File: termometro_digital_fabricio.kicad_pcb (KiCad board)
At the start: 2 copper layers, 100 x 100 mm, 30 parts, among them J1 Conn_01x01_Pin, SW1 SW_Push, U1 MT3608, U2 L7805, U3 LM35-LP, U4 ICL7107CPL, U5 ICL7660, U7 18650

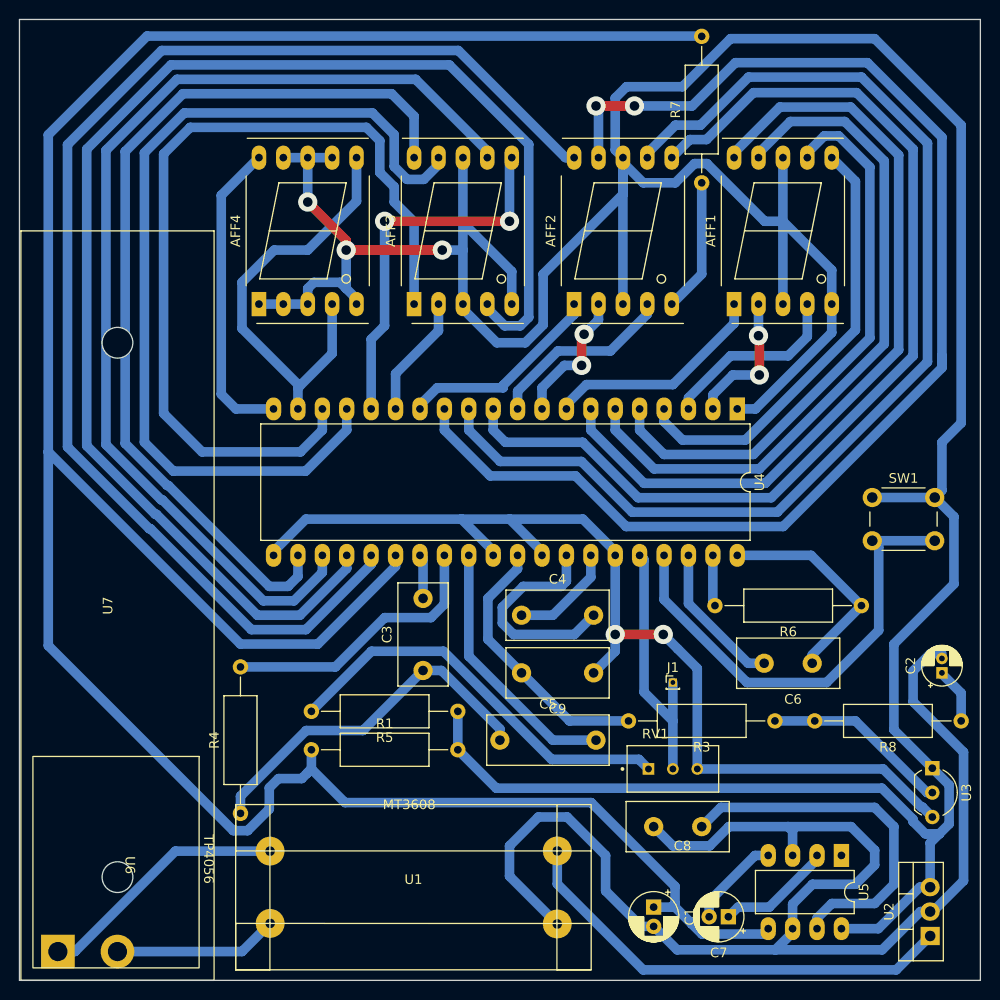
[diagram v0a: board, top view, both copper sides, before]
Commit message: Uploading files
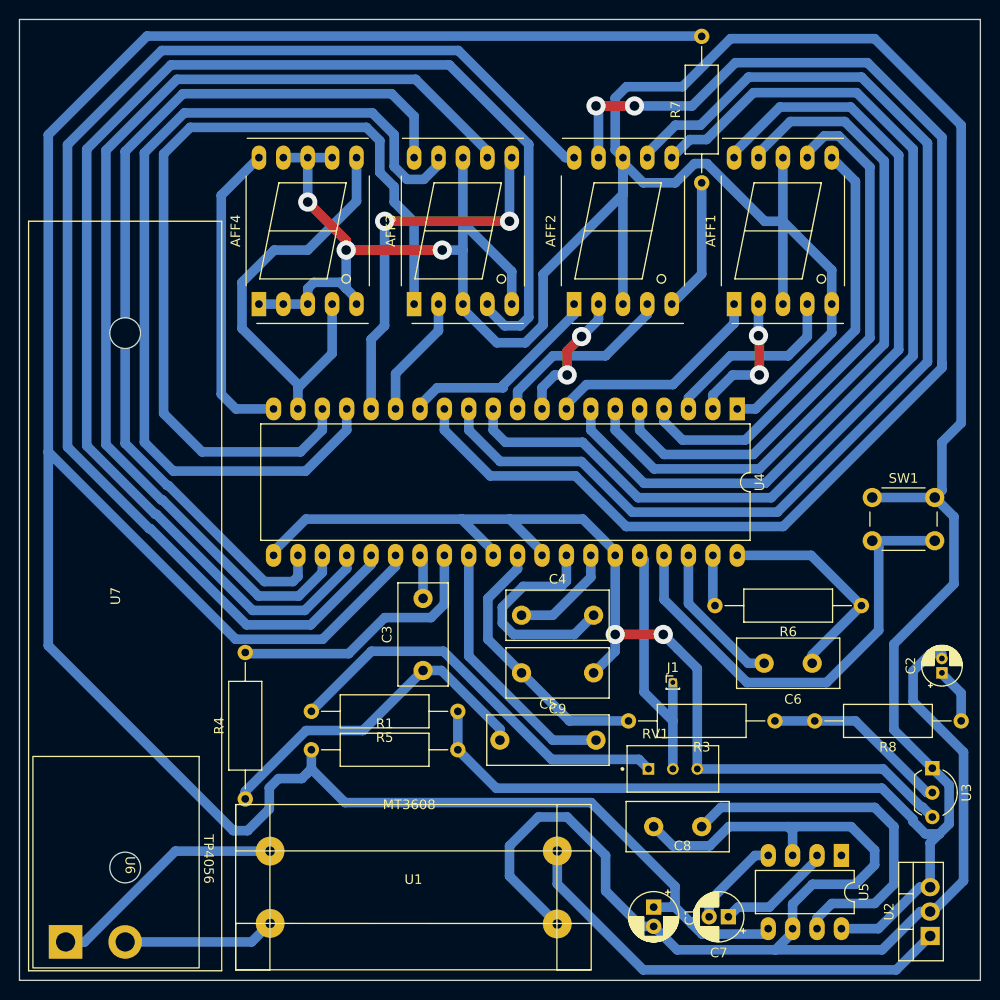
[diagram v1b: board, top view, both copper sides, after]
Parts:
- moved R4 1.58 mm to (154.5, 127.1)
- moved U7 1.28 mm to (142.0, 70.0)
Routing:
- net Net-(C3-Pad1): track 37.9 -> 36.2 mm
- net Net-(U1-IN-): track 17.1 -> 15.9 mm
- net Net-(U1-IN+): track 26.4 -> 25.2 mm
- net Net-(U4-BUFF): track 29.0 -> 27.9 mm
- net Net-(AFF2-f): track 136.3 -> 135.5 mm
- net VEE: track 275.0 -> 274.4 mm
